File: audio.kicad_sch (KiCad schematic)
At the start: 46 parts, among them J15 SPEAKER, J4 SPEAKER, U6 WM8960, U7 MAX9814, Y2 12.288M

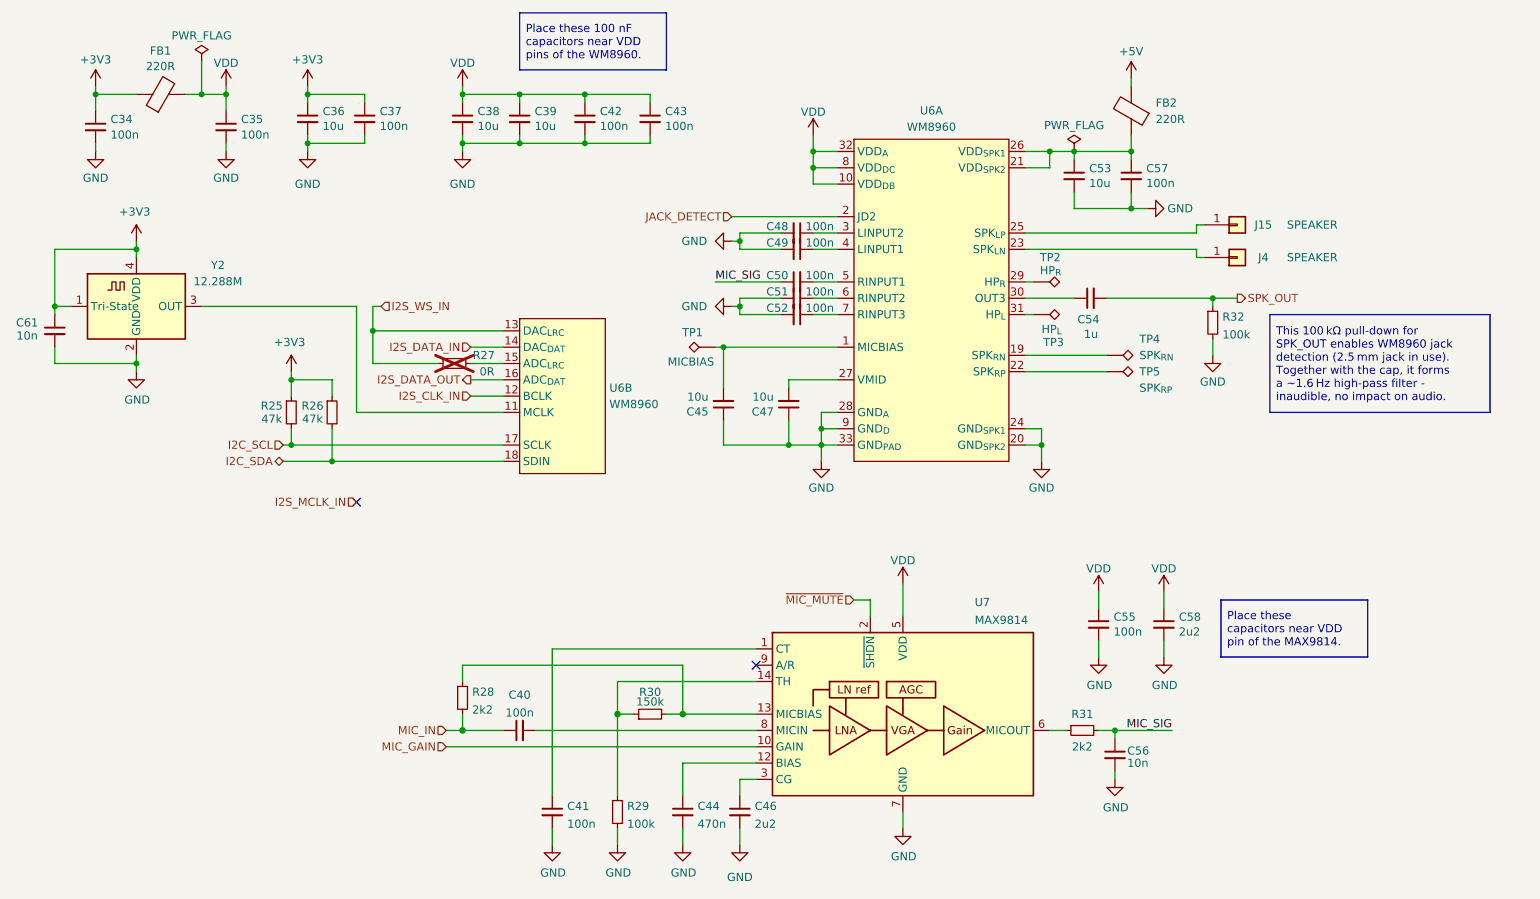
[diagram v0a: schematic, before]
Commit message: Replaced WM8960 to the newer TLV320AIC3100
WM8960 is obsolete, so this change is needed.
Fixes #29
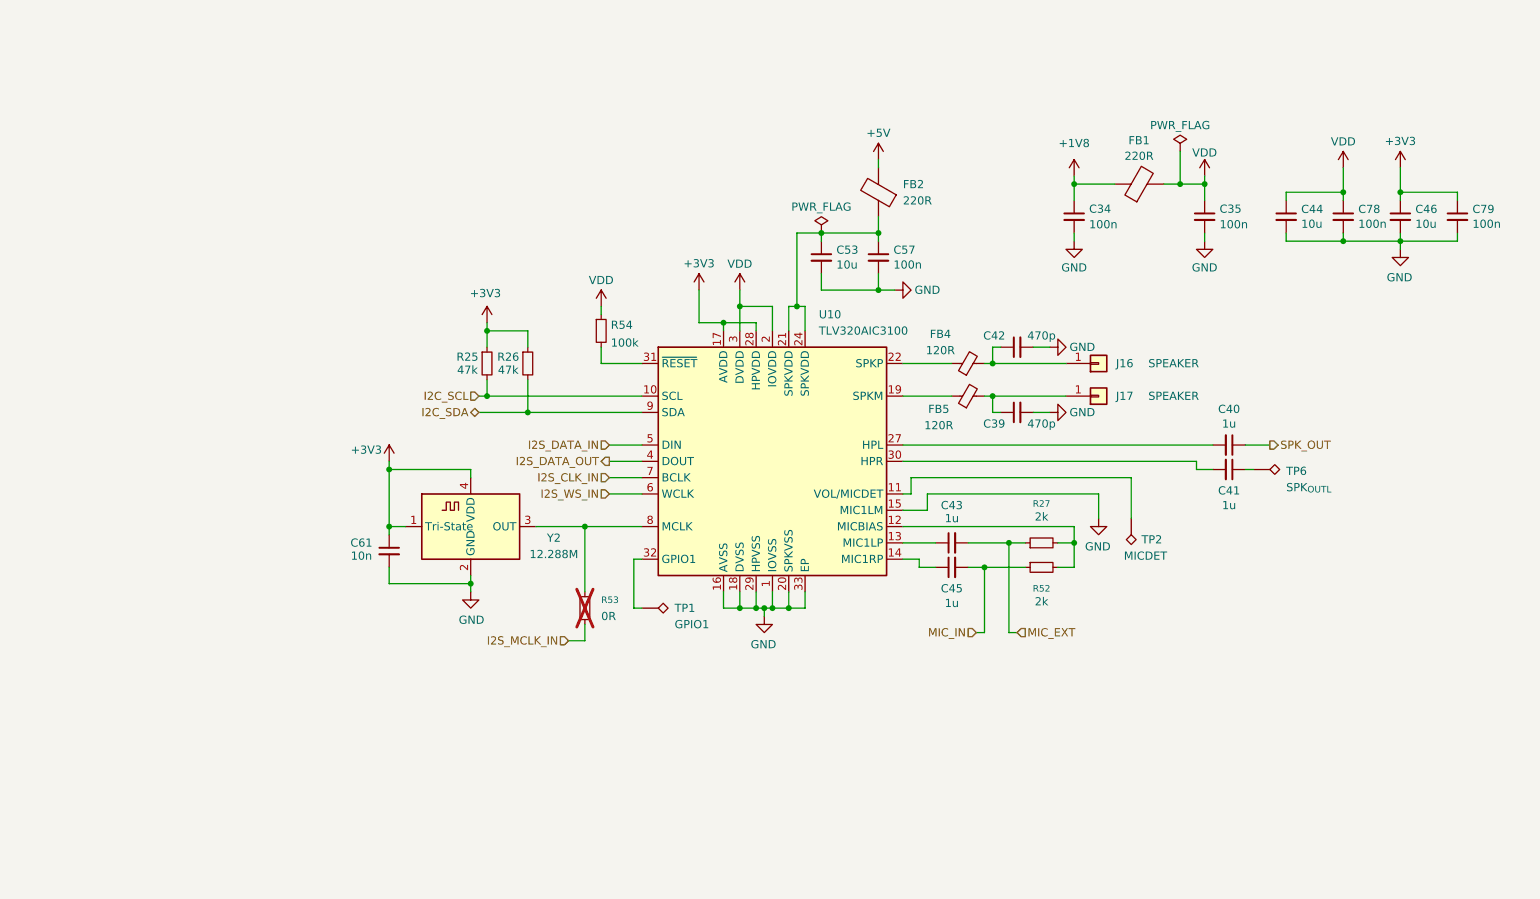
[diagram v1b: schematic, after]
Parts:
- removed C36, C38, C47: 10u, Capacitor_SMD:C_0402_1005Metric, symbol Device:C_Small
- removed C37, C48, C49, C50, C51, C52, C55: 100n, Capacitor_SMD:C_0402_1005Metric, symbol Device:C_Small
- removed C54: 1u, Capacitor_SMD:C_0402_1005Metric, symbol Device:C_Small
- removed C56: 10n, Capacitor_SMD:C_0402_1005Metric, symbol Device:C_Small
- removed C58: 2u2, Capacitor_SMD:C_0402_1005Metric, symbol Device:C_Small
- removed J15, J4: SPEAKER, TestPoint:TestPoint_Pad_D4.0mm, symbol Connector_Generic:Conn_01x01
- removed R28, R31: 2k2, Resistor_SMD:R_0402_1005Metric, symbol Device:R_Small
- removed R29, R32: 100k, Resistor_SMD:R_0402_1005Metric, symbol Device:R_Small
- removed R30: 150k, Resistor_SMD:R_0402_1005Metric, symbol Device:R_Small
- removed TP3: HP_{L}, TestPoint:TestPoint_Pad_D1.0mm, symbol Connector:TestPoint_Alt
- removed TP4: SPK_{RN}, TestPoint:TestPoint_Pad_D1.0mm, symbol Connector:TestPoint_Alt
- removed TP5: SPK_{RP}, TestPoint:TestPoint_Pad_D1.0mm, symbol Connector:TestPoint_Alt
- removed U6: WM8960, Package_DFN_QFN:QFN-32-1EP_5x5mm_P0.5mm_EP3.6x3.6mm_ThermalVias, symbol WM8960:WM8960
- removed U7: MAX9814, Package_DFN_QFN:DFN-14-1EP_3x3mm_P0.4mm_EP1.78x2.35mm, symbol Amplifier_Audio:MAX9814
- added C78, C79: 100n, Capacitor_SMD:C_0402_1005Metric, symbol Device:C_Small
- added FB4, FB5: 120R, Inductor_SMD:L_0805_2012Metric, symbol Device:FerriteBead_Small
- added J16, J17: SPEAKER, TestPoint:TestPoint_Pad_D4.0mm, symbol Connector_Generic:Conn_01x01
- added R52: 2k, Resistor_SMD:R_0402_1005Metric, symbol Device:R_Small
- added R53: 0R, Resistor_SMD:R_0402_1005Metric, symbol Device:R_Small
- added R54: 100k, Resistor_SMD:R_0402_1005Metric, symbol Device:R_Small
- added TP6: SPK_{OUTL}, TestPoint:TestPoint_Pad_D1.0mm, symbol Connector:TestPoint_Alt
- added U10: TLV320AIC3100, Package_DFN_QFN:VQFN-32-1EP_5x5mm_P0.5mm_EP3.5x3.5mm, symbol Audio:TLV320AIC3100
- C39: value 10u -> 470p; LCSC C15525 -> C106259; MPN CL05A106MQ5NUNC -> CC0402JRNPO9BN471; PN 187-CL05A106MQ5NUNC -> (none)
- C40, C41, C43: value 100n -> 1u; LCSC C1525 -> CL05A105KA5NQNC; MPN CL05B104KO5NNNC -> CL05A105KA5NQNC; PN 187-CL05B104KO5NNNC -> (none)
- C42: value 100n -> 470p; LCSC C1525 -> C106259; MPN CL05B104KO5NNNC -> CC0402JRNPO9BN471; PN 187-CL05B104KO5NNNC -> (none)
- C44: value 470n -> 10u; LCSC C2895720 -> C15525; MPN CL05B474KP5NNNC -> CL05A106MQ5NUNC; PN 187-CL05B474KP5NNNC -> 187-CL05A106MQ5NUNC
- C45: value 10u -> 1u; LCSC C15525 -> CL05A105KA5NQNC; MPN CL05A106MQ5NUNC -> CL05A105KA5NQNC; PN 187-CL05A106MQ5NUNC -> (none)
- C46: value 2u2 -> 10u; LCSC C170151 -> C15525; MPN CL05A225KO5NQNC -> CL05A106MQ5NUNC; PN 187-CL05A225KO5NQNC -> 187-CL05A106MQ5NUNC
- R27: value 0R -> 2k; LCSC (none) -> C4109; PN (none) -> 0402WGF2001TCE; now fitted; now in the parts list
- TP1: value MICBIAS -> GPIO1
- TP2: value HP_{R} -> MICDET
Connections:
- net +3V3: now also C46.1, C79.1, U10.17 (AVDD), U10.28 (HPVDD); no longer C34.1, FB1.1
- net GND: now also C78.2, C79.2, U10.1 (IOVSS), U10.15 (MIC1LM), U10.16 (AVSS), U10.18 (DVSS), U10.20 (SPKVSS), U10.25 (SPKVSS), U10.29 (HPVSS), U10.33 (EP); no longer C41.2, C43.2, C45.1
- net I2C_SCL: now also U10.10 (SCL)
- net I2C_SDA: now also U10.9 (SDA)
- net I2S_CLK_IN: now also U10.7 (BCLK)
- net I2S_DATA_IN: now also U10.5 (DIN)
- net I2S_DATA_OUT: now also U10.4 (DOUT)
- net I2S_MCLK_IN: now also R53.2
- net I2S_WS_IN: now also U10.6 (WCLK); no longer R27.2
- net MIC_IN: now also C45.2, R52.1; no longer C40.1
- net SPK_OUT: now also C40.1
- net VDD: now also C44.1, C78.1, R54.1, U10.2 (IOVDD), U10.3 (DVDD); no longer C39.1, C42.1, C43.1
- net at C40.2: now also U10.27 (HPL)
- net at Y2.3 (OUT): now also R53.1, U10.8 (MCLK)
- net MIC_EXT: now reaches R27.1
- net MIC_EXT: now also C43.2
- net at C53.1, C57.1, FB2.1: now also U10.21 (SPKVDD), U10.24 (SPKVDD)
- net at TP1.1: now also U10.32 (GPIO1); no longer C45.2
- net at C41.1: now also TP6.1
- net at TP2.1: now also U10.11 (VOL/MICDET)
- new net: R27.2, R52.2, U10.12 (MICBIAS)
- new net: C43.1, U10.13 (MIC1LP)
- new net: C42.1, FB4.2, J16.1 (Pin_1)
- new net: R54.2, U10.31 (~{RESET})
- new net: C41.2, U10.30 (HPR)
- new net: C39.1, FB5.2, J17.1 (Pin_1)
- new net: C45.1, U10.14 (MIC1RP)
- new net: FB5.1, U10.19 (SPKM), U10.23 (SPKM)
- new net: FB4.1, U10.22 (SPKP), U10.26 (SPKP)
- new net +1V8: C34.1, FB1.1
- no-connect marks 2 -> 0
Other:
- moved on the sheet: C34, C35, C53, C57, C61, FB1, FB2, R25, R26, Y2
